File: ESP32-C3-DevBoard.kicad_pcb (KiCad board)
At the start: 2 copper layers, 25.4 x 26.7 mm, 19 parts, among them J1 USB_C_Receptacle_USB2.0, J2 Conn_01x10, J3 Conn_01x10, SW1 SW_Push, SW2 SW_Push, U1 ESP32-C3-WROOM-02, U2 AMS1117-3.3

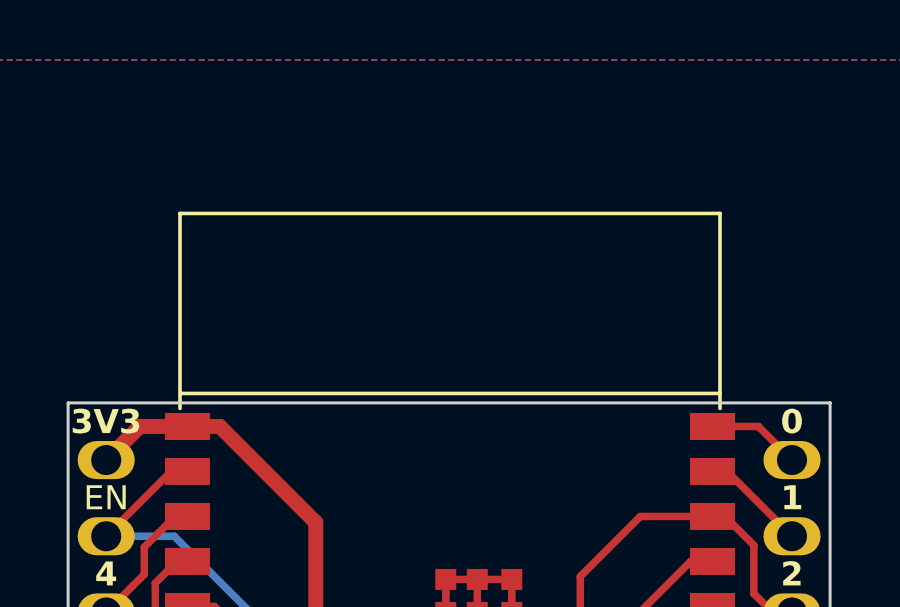
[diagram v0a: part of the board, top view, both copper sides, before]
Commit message: Add files via upload
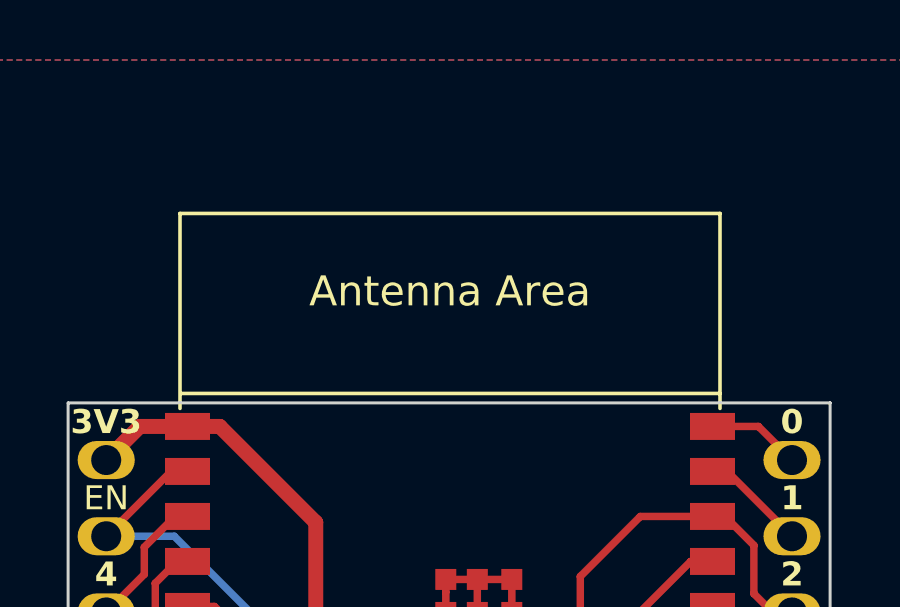
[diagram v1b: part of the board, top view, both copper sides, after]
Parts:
- H1, H2: value MountingHole -> ToolingHole
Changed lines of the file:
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@@
   (title_block
     (title "ESP32-C3 Development Board")
-    (rev "v1.0.0")
+    (rev "v1.0.1")
   )
   (layers
@@
     (pad "2" smd roundrect (at 0.51 0) (size 0.54 0.64) (layers "F.Cu" "F.Paste" "F.Mask") (roundrect_rratio 0.25)
       (net 15 "/IO2") (pintype "passive"))
-    (model "${KICAD6_3DMODEL_DIR}/Resistor_SMD.3dshapes/R_0402_1005Metric.wrl"
+    (model "${KICAD7_3DMODEL_DIR}/Resistor_SMD.3dshapes/R_0402_1005Metric.wrl"
       (offset (xyz 0 0 0))
       (scale (xyz 1 1 1))
@@
     (pad "2" smd roundrect (at 0.51 0 180) (size 0.54 0.64) (layers "F.Cu" "F.Paste" "F.Mask") (roundrect_rratio 0.25)
       (net 6 "/IO8") (pintype "passive"))
-    (model "${KICAD6_3DMODEL_DIR}/Resistor_SMD.3dshapes/R_0402_1005Metric.wrl"
+    (model "${KICAD7_3DMODEL_DIR}/Resistor_SMD.3dshapes/R_0402_1005Metric.wrl"
       (offset (xyz 0 0 0))
       (scale (xyz 1 1 1))
@@
     (pad "2" smd roundrect (at 0.95 0 270) (size 1 1.45) (layers "F.Cu" "F.Paste" "F.Mask") (roundrect_rratio 0.25)
       (net 8 "GND") (pintype "passive"))
-    (model "${KICAD6_3DMODEL_DIR}/Capacitor_SMD.3dshapes/C_0805_2012Metric.wrl"
+    (model "${KICAD7_3DMODEL_DIR}/Capacitor_SMD.3dshapes/C_0805_2012Metric.wrl"
       (offset (xyz 0 0 0))
       (scale (xyz 1 1 1))
@@
     (pad "2" smd roundrect (at 0.48 0) (size 0.56 0.62) (layers "F.Cu" "F.Paste" "F.Mask") (roundrect_rratio 0.25)
       (net 18 "+3V3") (pintype "passive"))
-    (model "${KICAD6_3DMODEL_DIR}/Capacitor_SMD.3dshapes/C_0402_1005Metric.wrl"
+    (model "${KICAD7_3DMODEL_DIR}/Capacitor_SMD.3dshapes/C_0402_1005Metric.wrl"
       (offset (xyz 0 0 0))
       (scale (xyz 1 1 1))
@@
     (pad "2" smd roundrect (at 0.51 0) (size 0.54 0.64) (layers "F.Cu" "F.Paste" "F.Mask") (roundrect_rratio 0.25)
       (net 8 "GND") (pintype "passive"))
-    (model "${KICAD6_3DMODEL_DIR}/Resistor_SMD.3dshapes/R_0402_1005Metric.wrl"
+    (model "${KICAD7_3DMODEL_DIR}/Resistor_SMD.3dshapes/R_0402_1005Metric.wrl"
       (offset (xyz 0 0 0))
       (scale (xyz 1 1 1))
@@
         (effects (font (size 1 1) (thickness 0.15)))
     )
-    (fp_text value "MountingHole" (at 0 3.2) (layer "F.Fab")
+    (fp_text value "ToolingHole" (at 0 3.2) (layer "F.Fab")
         (effects (font (size 1 1) (thickness 0.15)))
     )
@@
         (effects (font (size 1 1) (thickness 0.15)))
     )
-    (fp_text user "Antenna Area" (at 0 -10.4) (layer "F.SilkS") hide
+    (fp_text user "Antenna Area" (at 0 -10.4) (layer "F.SilkS")
         (effects (font (size 1 1) (thickness 0.15)))
     )
@@
     (pad "2" smd roundrect (at 0.95 0 180) (size 1 1.45) (layers "F.Cu" "F.Paste" "F.Mask") (roundrect_rratio 0.25)
       (net 19 "+5V") (pintype "passive"))
-    (model "${KICAD6_3DMODEL_DIR}/Capacitor_SMD.3dshapes/C_0805_2012Metric.wrl"
+    (model "${KICAD7_3DMODEL_DIR}/Capacitor_SMD.3dshapes/C_0805_2012Metric.wrl"
       (offset (xyz 0 0 0))
       (scale (xyz 1 1 1))
@@
     (pad "2" smd roundrect (at 0.48 0) (size 0.56 0.62) (layers "F.Cu" "F.Paste" "F.Mask") (roundrect_rratio 0.25)
       (net 8 "GND") (pintype "passive"))
-    (model "${KICAD6_3DMODEL_DIR}/Capacitor_SMD.3dshapes/C_0402_1005Metric.wrl"
+    (model "${KICAD7_3DMODEL_DIR}/Capacitor_SMD.3dshapes/C_0402_1005Metric.wrl"
       (offset (xyz 0 0 0))
       (scale (xyz 1 1 1))
@@
         (effects (font (size 1 1) (thickness 0.15)))
     )
-    (fp_text value "MountingHole" (at 0 3.2) (layer "F.Fab")
+    (fp_text value "ToolingHole" (at 0 3.2) (layer "F.Fab")
         (effects (font (size 1 1) (thickness 0.15)))
     )
@@
     (pad "2" smd roundrect (at 1.05 0) (size 0.6 0.45) (layers "F.Cu" "F.Paste" "F.Mask") (roundrect_rratio 0.25)
       (net 20 "VBUS") (pinfunction "A") (pintype "passive"))
-    (model "${KICAD6_3DMODEL_DIR}/Diode_SMD.3dshapes/D_SOD-323.wrl"
+    (model "${KICAD7_3DMODEL_DIR}/Diode_SMD.3dshapes/D_SOD-323.wrl"
       (offset (xyz 0 0 0))
       (scale (xyz 1 1 1))
@@
     (pad "2" smd roundrect (at 0.51 0 180) (size 0.54 0.64) (layers "F.Cu" "F.Paste" "F.Mask") (roundrect_rratio 0.25)
       (net 1 "/EN") (pintype "passive"))
-    (model "${KICAD6_3DMODEL_DIR}/Resistor_SMD.3dshapes/R_0402_1005Metric.wrl"
+    (model "${KICAD7_3DMODEL_DIR}/Resistor_SMD.3dshapes/R_0402_1005Metric.wrl"
       (offset (xyz 0 0 0))
       (scale (xyz 1 1 1))
@@
     (pad "2" smd roundrect (at 0.51 0 180) (size 0.54 0.64) (layers "F.Cu" "F.Paste" "F.Mask") (roundrect_rratio 0.25)
       (net 23 "Net-(J1-CC2)") (pintype "passive"))
-    (model "${KICAD6_3DMODEL_DIR}/Resistor_SMD.3dshapes/R_0402_1005Metric.wrl"
+    (model "${KICAD7_3DMODEL_DIR}/Resistor_SMD.3dshapes/R_0402_1005Metric.wrl"
       (offset (xyz 0 0 0))
       (scale (xyz 1 1 1))
@@
     (pad "3" smd rect (at -1.95 1.5 180) (size 1.3 0.9) (layers "F.Cu" "F.Paste" "F.Mask")
       (net 19 "+5V") (pinfunction "VI") (pintype "power_in"))
-    (model "${KICAD6_3DMODEL_DIR}/Package_TO_SOT_SMD.3dshapes/SOT-89-3.wrl"
+    (model "${KICAD7_3DMODEL_DIR}/Package_TO_SOT_SMD.3dshapes/SOT-89-3.wrl"
       (offset (xyz 0 0 0))
       (scale (xyz 1 1 1))
@@
     (pad "10" thru_hole oval (at 0 -22.86 180) (size 1.905 1.27) (drill 1) (layers "*.Cu" "*.Mask")
       (net 8 "GND") (pinfunction "Pin_10") (pintype "passive"))
-    (model "${KICAD6_3DMODEL_DIR}/Connector_PinHeader_2.54mm.3dshapes/PinHeader_1x10_P2.54mm_Vertical.wrl"
+    (model "${KICAD7_3DMODEL_DIR}/Connector_PinHeader_2.54mm.3dshapes/PinHeader_1x10_P2.54mm_Vertical.wrl"
       (offset (xyz 0 0 0))
       (scale (xyz 1 1 1))
@@
     (pad "10" thru_hole oval (at 0 -22.86 180) (size 1.905 1.27) (drill 1) (layers "*.Cu" "*.Mask")
       (net 8 "GND") (pinfunction "Pin_10") (pintype "passive"))
-    (model "${KICAD6_3DMODEL_DIR}/Connector_PinHeader_2.54mm.3dshapes/PinHeader_1x10_P2.54mm_Vertical.wrl"
-      (offset (xyz 0 0 0))
-      (scale (xyz 1 1 1))
+    (model "${KICAD7_3DMODEL_DIR}/Connector_PinHeader_2.54mm.3dshapes/PinHeader_1x10_P2.54mm_Vertical.wrl"
+      (offset (xyz 0 0 0))
+      (scale (xyz 1 1 1))

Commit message: Add Tooling Hole Library
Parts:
- H1, H2: footprint MountingHole:MountingHole_2.2mm_M2 -> Tooling_Hole:Tooling_Hole
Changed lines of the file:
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@@
     )
   )
-  (footprint "MountingHole:MountingHole_2.2mm_M2" (layer "F.Cu")
+  (footprint "Tooling_Hole:Tooling_Hole" (layer "F.Cu")
     (at 137.16 113.665)
-    (descr "Mounting Hole 2.2mm, no annular, M2")
-    (tags "mounting hole 2.2mm no annular m2")
     (property "Sheetfile" "ESP32-C3-DevBoard.kicad_sch")
     (property "Sheetname" "")
@@
     (property "ki_description" "Mounting Hole without connection")
     (property "ki_keywords" "mounting hole")
-    (attr exclude_from_pos_files exclude_from_bom allow_missing_courtyard)
-    (fp_text reference "H1" (at 0 -3.2) (layer "F.SilkS") hide
-        (effects (font (size 1 1) (thickness 0.15)))
-    )
-    (fp_text value "ToolingHole" (at 0 3.2) (layer "F.Fab")
-        (effects (font (size 1 1) (thickness 0.15)))
-    )
-    (fp_text user "${REFERENCE}" (at 0 0) (layer "F.Fab")
+    (attr exclude_from_bom)
+    (fp_text reference "H1" (at 0 -1.27 unlocked) (layer "F.SilkS") hide
+        (effects (font (size 1 1) (thickness 0.15)))
+    )
+    (fp_text value "ToolingHole" (at 0 1 unlocked) (layer "F.Fab")
+        (effects (font (size 1 1) (thickness 0.15)))
+    )
+    (fp_text user "${REFERENCE}" (at 0 2.5 unlocked) (layer "F.Fab")
         (effects (font (size 1 1) (thickness 0.15)))
     )
@@
     )
   )
-  (footprint "MountingHole:MountingHole_2.2mm_M2" (layer "F.Cu")
+  (footprint "Tooling_Hole:Tooling_Hole" (layer "F.Cu")
     (at 154.94 113.665)
-    (descr "Mounting Hole 2.2mm, no annular, M2")
-    (tags "mounting hole 2.2mm no annular m2")
     (property "Sheetfile" "ESP32-C3-DevBoard.kicad_sch")
     (property "Sheetname" "")
@@
     (property "ki_description" "Mounting Hole without connection")
     (property "ki_keywords" "mounting hole")
-    (attr exclude_from_pos_files exclude_from_bom allow_missing_courtyard)
-    (fp_text reference "H2" (at 0 -3.2) (layer "F.SilkS") hide
-        (effects (font (size 1 1) (thickness 0.15)))
-    )
-    (fp_text value "ToolingHole" (at 0 3.2) (layer "F.Fab")
-        (effects (font (size 1 1) (thickness 0.15)))
-    )
-    (fp_text user "${REFERENCE}" (at 0 0) (layer "F.Fab")
-        (effects (font (size 1 1) (thickness 0.15)))
-    )
+    (attr exclude_from_bom)
+    (fp_text reference "H2" (at 0 -1.27 unlocked) (layer "F.SilkS") hide
+        (effects (font (size 1 1) (thickness 0.15)))
+    )
+    (fp_text value "ToolingHole" (at 0 1 unlocked) (layer "F.Fab")
+        (effects (font (size 1 1) (thickness 0.15)))
+    )
+    (fp_text user "${REFERENCE}" (at 0 2.5 unlocked) (layer "F.Fab")
+        (effects (font (size 1 1) (thickness 0.15)))
+    )

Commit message: Add files via upload
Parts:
- C2: value 10uF -> 22uF
- R1, R2: value 5.1KΩ -> 5.1kΩ
- R3, R4, R5: value 10K -> 10kΩ
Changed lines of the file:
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@@
         (effects (font (size 1 1) (thickness 0.15)))
     )
-    (fp_text value "10K" (at 0 1.17) (layer "F.Fab")
+    (fp_text value "10kΩ" (at 0 1.17) (layer "F.Fab")
         (effects (font (size 1 1) (thickness 0.15)))
     )
@@
         (effects (font (size 1 1) (thickness 0.15)))
     )
-    (fp_text value "10K" (at 0 1.17) (layer "F.Fab")
+    (fp_text value "10kΩ" (at 0 1.17) (layer "F.Fab")
         (effects (font (size 1 1) (thickness 0.15)))
     )
@@
     (descr "Capacitor SMD 0805 (2012 Metric), square (rectangular) end terminal, IPC_7351 nominal, (Body size source: IPC-SM-782 page 76, https://www.pcb-3d.com/wordpress/wp-content/uploads/ipc-sm-782a_amendment_1_and_2.pdf, https://docs.google.com/spreadsheets/d/1BsfQQcO9C6DZCsRaXUlFlo91Tg2WpOkGARC1WS5S8t0/edit?usp=sharing), generated with kicad-footprint-generator")
     (tags "capacitor")
-    (property "LCSC" "C15850")
+    (property "LCSC" "C45783")
     (property "Sheetfile" "ESP32-C3-DevBoard.kicad_sch")
     (property "Sheetname" "")
@@
         (effects (font (size 1 1) (thickness 0.15)))
     )
-    (fp_text value "10uF" (at 0 1.68 90) (layer "F.Fab")
+    (fp_text value "22uF" (at 0 1.68 90) (layer "F.Fab")
         (effects (font (size 1 1) (thickness 0.15)))
     )
@@
         (effects (font (size 1 1) (thickness 0.15)))
     )
-    (fp_text value "5.1KΩ" (at 0 1.17) (layer "F.Fab")
+    (fp_text value "5.1kΩ" (at 0 1.17) (layer "F.Fab")
         (effects (font (size 1 1) (thickness 0.15)))
     )
@@
         (effects (font (size 1 1) (thickness 0.15)))
     )
-    (fp_text value "10K" (at 0 1.17) (layer "F.Fab")
+    (fp_text value "10kΩ" (at 0 1.17) (layer "F.Fab")
         (effects (font (size 1 1) (thickness 0.15)))
     )
@@
         (effects (font (size 1 1) (thickness 0.15)))
     )
-    (fp_text value "5.1KΩ" (at 0 1.17) (layer "F.Fab")
-        (effects (font (size 1 1) (thickness 0.15)))
-    )
+    (fp_text value "5.1kΩ" (at 0 1.17) (layer "F.Fab")
+        (effects (font (size 1 1) (thickness 0.15)))
+    )
